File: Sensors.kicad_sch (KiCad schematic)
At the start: 20 parts, among them U3 INA226, U6 ADS333

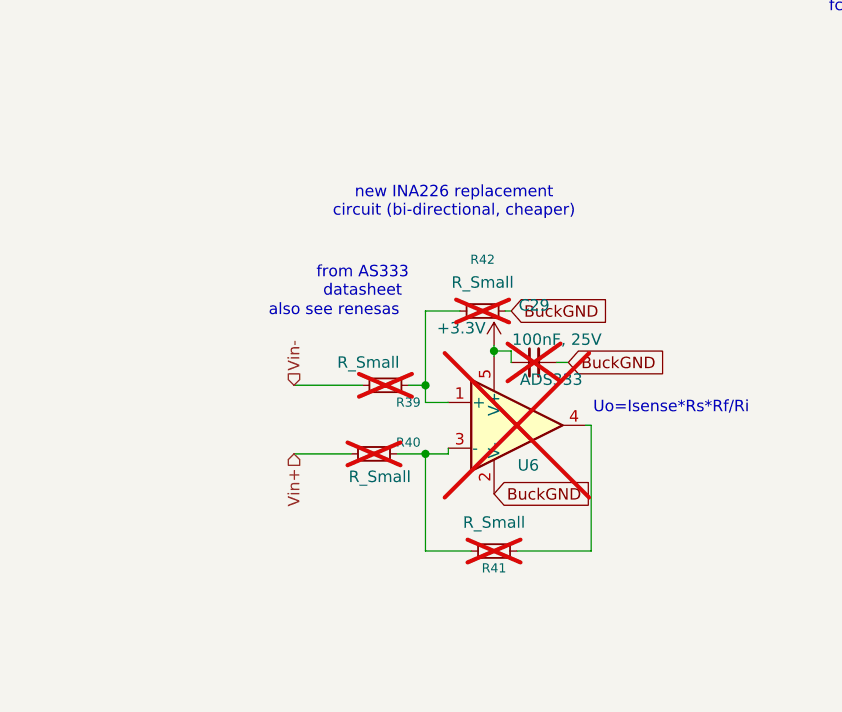
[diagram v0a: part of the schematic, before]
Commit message: opa current sense
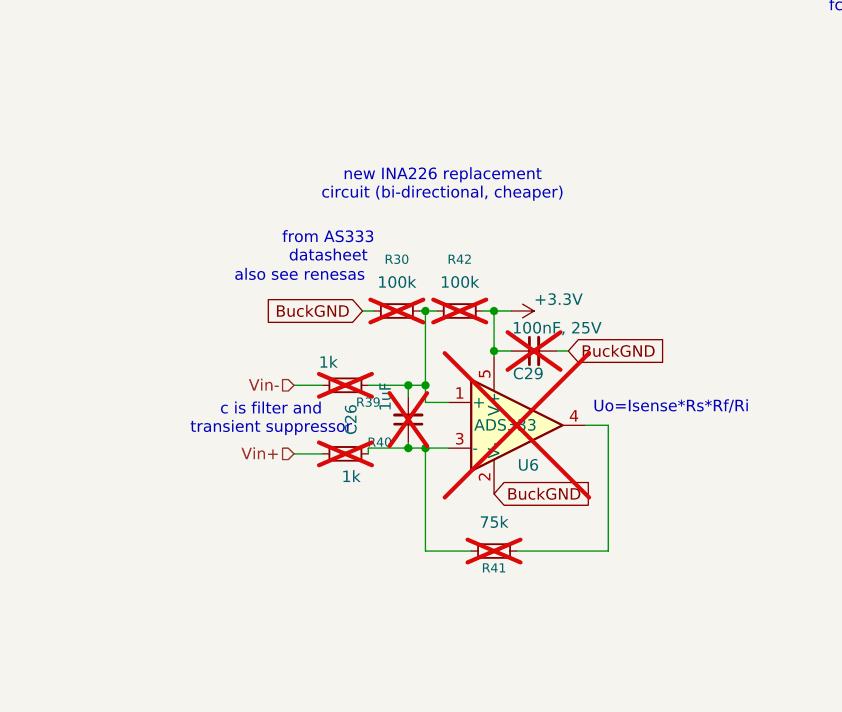
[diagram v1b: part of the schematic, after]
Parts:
- added C26: 1uF, Capacitor_SMD:C_0805_2012Metric, symbol Device:C_Small
- added R30: 100k, Resistor_SMD:R_0805_2012Metric, symbol Device:R_Small
- R39, R40: value R_Small -> 1k
- R41: value R_Small -> 75k
- R42: value R_Small -> 100k
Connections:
- net +3.3V: now also R42.2
- net BuckGND: now also R30.1; no longer R42.2
- net at R39.2, R42.1, U6.1 (+): now also C26.2, R30.2
- net at R40.2, R41.2, U6.3 (-): now also C26.1
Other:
- note added: "c is filter and transient suppressor"
- moved on the sheet: C29, R39, R40, R42
